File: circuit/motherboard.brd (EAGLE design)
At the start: 155.2 x 104.8 mm, 16 parts, among them J1 XF2L-2235-1, J2 XF2L-2235-1, T1 BC337

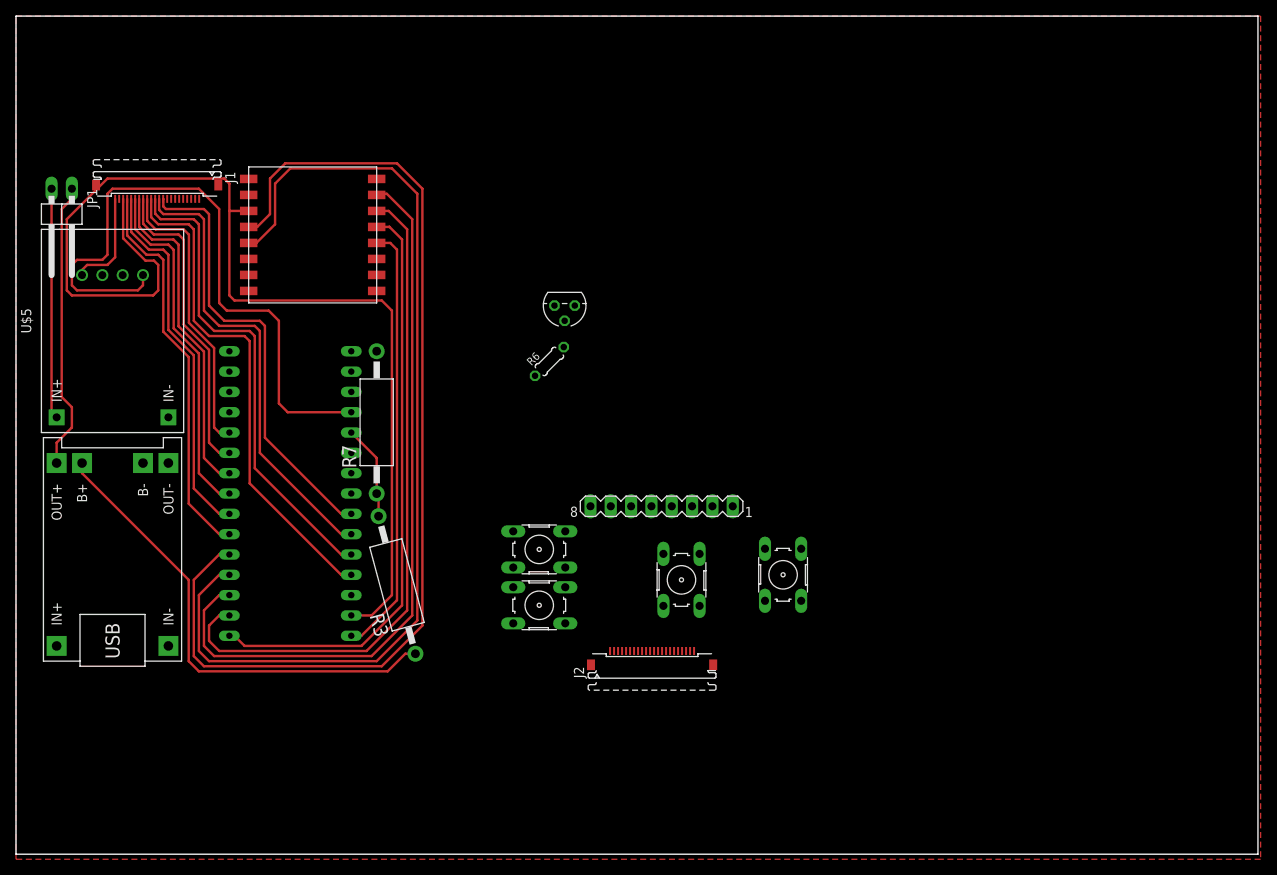
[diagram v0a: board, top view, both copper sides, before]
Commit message: Real life is gritty! - Etching at this point
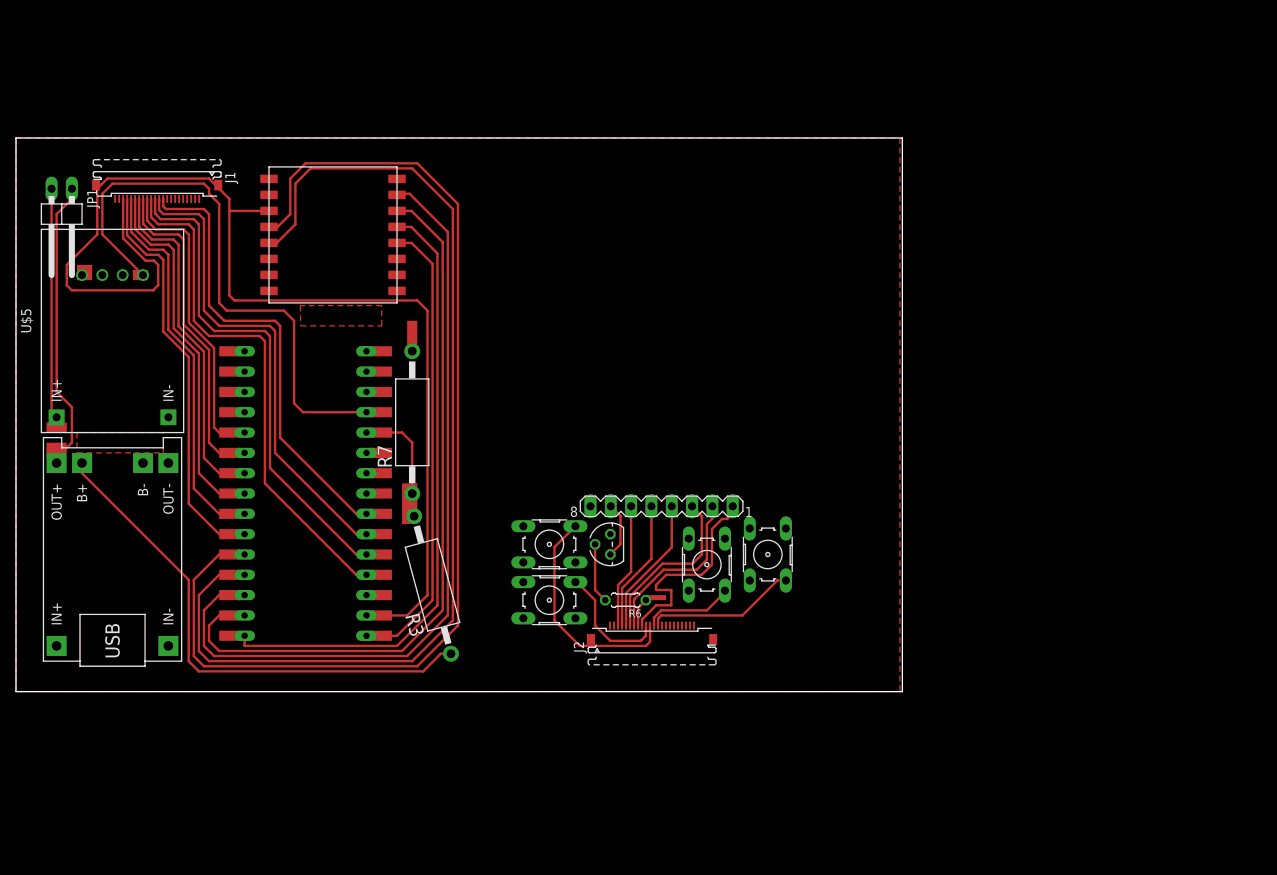
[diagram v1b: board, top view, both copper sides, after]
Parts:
- moved R6 31.3 mm to (83.8, 12.1), turned to 180 degrees
- moved T1 30.4 mm to (81.9, 19.1), turned to 90 degrees
- moved S2 29.5 mm to (74.3, 19.1), turned to 180 degrees
- moved S4 28.6 mm to (101.6, 17.8), turned to 90 degrees
- moved S3 21.6 mm to (94.0, 16.5), turned to 90 degrees
- moved S1 16.7 mm to (74.3, 12.1), turned to 180 degrees
- moved R3 4.45 mm to (59.7, 14.0)
- moved R7 4.45 mm to (57.1, 34.3)
- moved J2 3.18 mm to (87.6, 6.99)
- moved U$4 2.54 mm to (47.2, 57.7)
- moved U$1 1.91 mm to (41.3, 34.3)
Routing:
- net N$21: track 0.00 -> 28.4 mm
- net N$17: track 0.00 -> 26.4 mm
- net N$29: track 0.00 -> 22.7 mm
- net N$28: track 0.00 -> 21.3 mm
- net N$30: track 0.00 -> 18.8 mm
- net N$26: track 0.00 -> 17.7 mm
- net N$27: track 0.00 -> 17.3 mm
- net N$25: track 0.00 -> 15.6 mm
- net N$20: track 0.00 -> 15.3 mm
- net GND: track 12.7 -> 0.00 mm
- net N$22: track 0.00 -> 11.4 mm
- net +5V: track 81.1 -> 71.3 mm
- net N$14: track 0.00 -> 7.51 mm
- net N$6: track 92.4 -> 99.7 mm
- net N$5: track 84.8 -> 92.1 mm
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- added copper zone on layer 1, net N$18
- added copper zone on layer 1, net N$31
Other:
- board size 155.2 x 104.8 mm -> 110.8 x 69.2 mm
